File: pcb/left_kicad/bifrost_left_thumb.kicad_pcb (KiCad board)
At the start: 2 copper layers, 57.8 x 36.4 mm, 12 parts, among them J1 Conn_01x06, SW1 UNASSIGNED_41, SW2 UNASSIGNED_42, SW3 UNASSIGNED_43

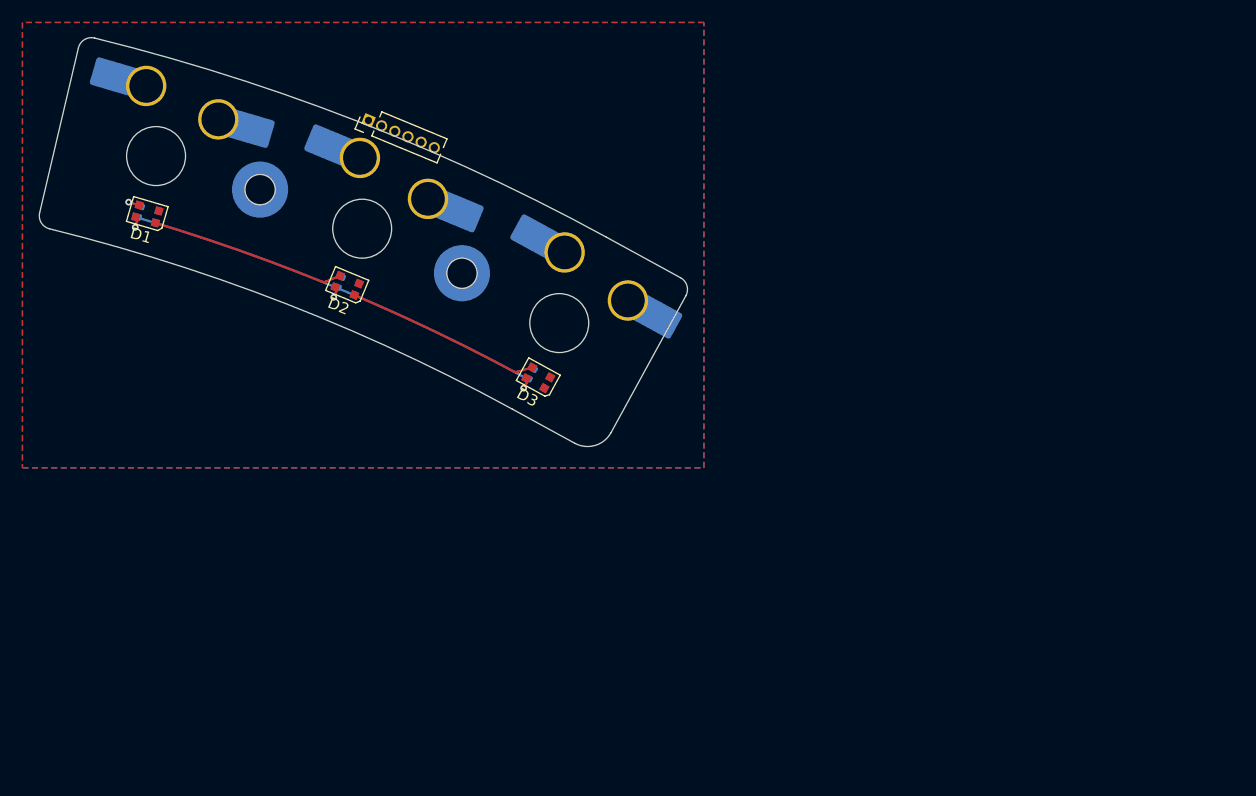
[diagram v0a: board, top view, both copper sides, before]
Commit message: Update PCB designs
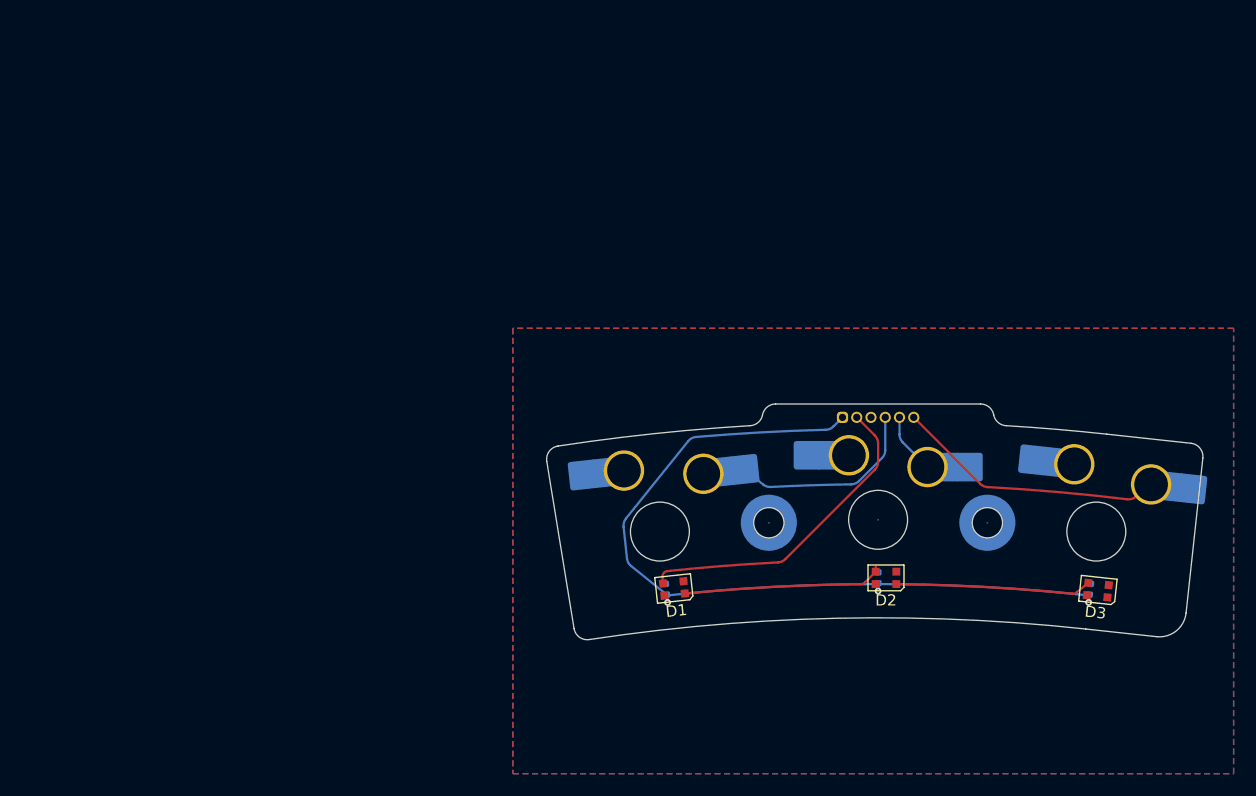
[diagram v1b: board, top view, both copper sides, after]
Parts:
- J1: moved to B.Cu
- SW1: value UNASSIGNED_41 -> 1U
- SW2: value UNASSIGNED_42 -> 1U
- SW3: value UNASSIGNED_43 -> 1U
- moved C1 57.7 mm to (120.0, 105.4), turned to 96.179 degrees
- moved D1 57.6 mm to (120.7, 105.3), turned to -173.821 degrees
- moved SW1 56.0 mm to (119.5, 100.3), turned to 6.179 degrees
- moved C2 54.7 mm to (138.9, 104.4), turned to 90 degrees
- moved D2 54.6 mm to (139.6, 104.4), turned to 180 degrees
- moved H1 54.2 mm to (129.2, 99.5), turned to -157.5 degrees
- moved C3 53.3 mm to (157.8, 105.4), turned to 83.821 degrees
- moved D3 53.3 mm to (158.5, 105.5), turned to 173.821 degrees
- moved SW2 52.8 mm to (138.9, 99.2), turned to 0 degrees
- moved H2 51.8 mm to (148.6, 99.5), turned to -157.5 degrees
- moved SW3 51.3 mm to (158.3, 100.3), turned to -6.179 degrees
- moved J1 49.8 mm to (135.7, 90.1), turned to -90 degrees
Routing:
- net RGB_PWR: track 43.5 -> 73.7 mm
- net RGB: track 1.23 -> 28.9 mm, vias 1 -> 0
- net PIN_T3: track 0.00 -> 24.2 mm
- net PIN_T1: track 0.00 -> 17.4 mm
- net PIN_T2: track 0.00 -> 5.41 mm
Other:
- board size 57.8 x 36.4 mm -> 58.5 x 21 mm
